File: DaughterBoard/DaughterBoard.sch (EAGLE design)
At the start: 6 parts

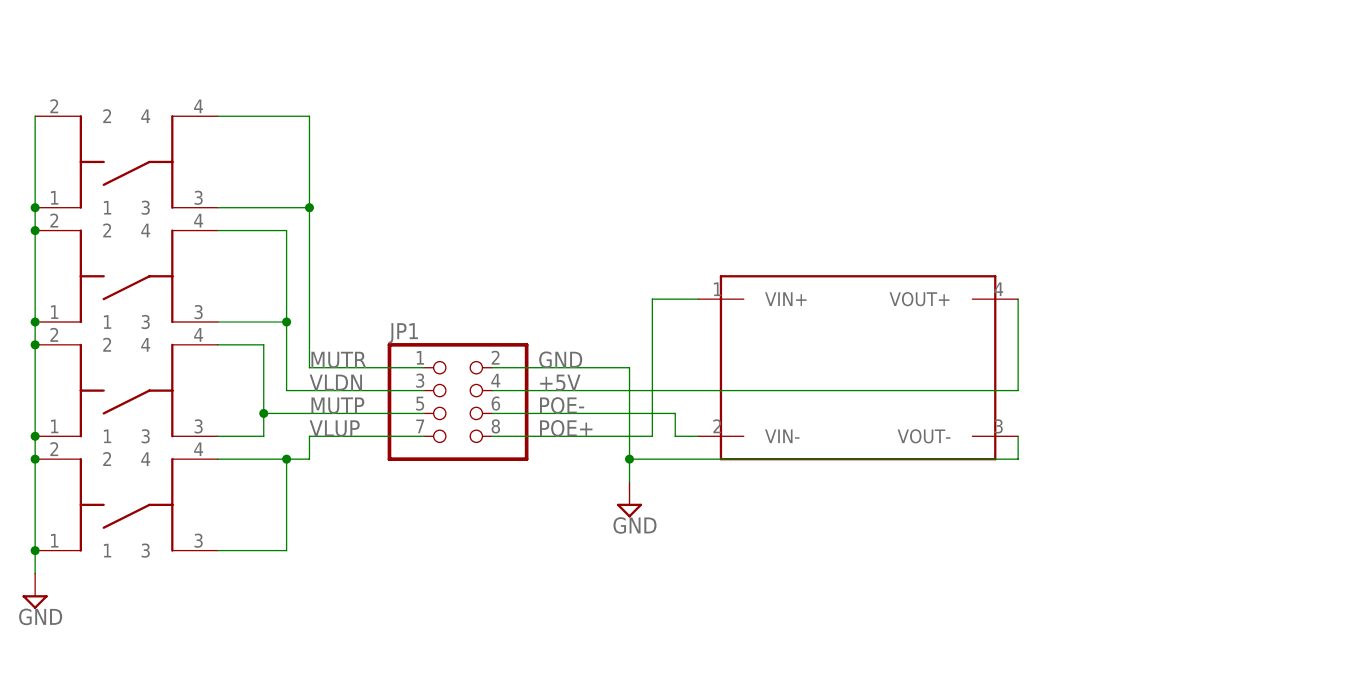
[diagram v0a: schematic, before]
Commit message: Finished modified daughterboard
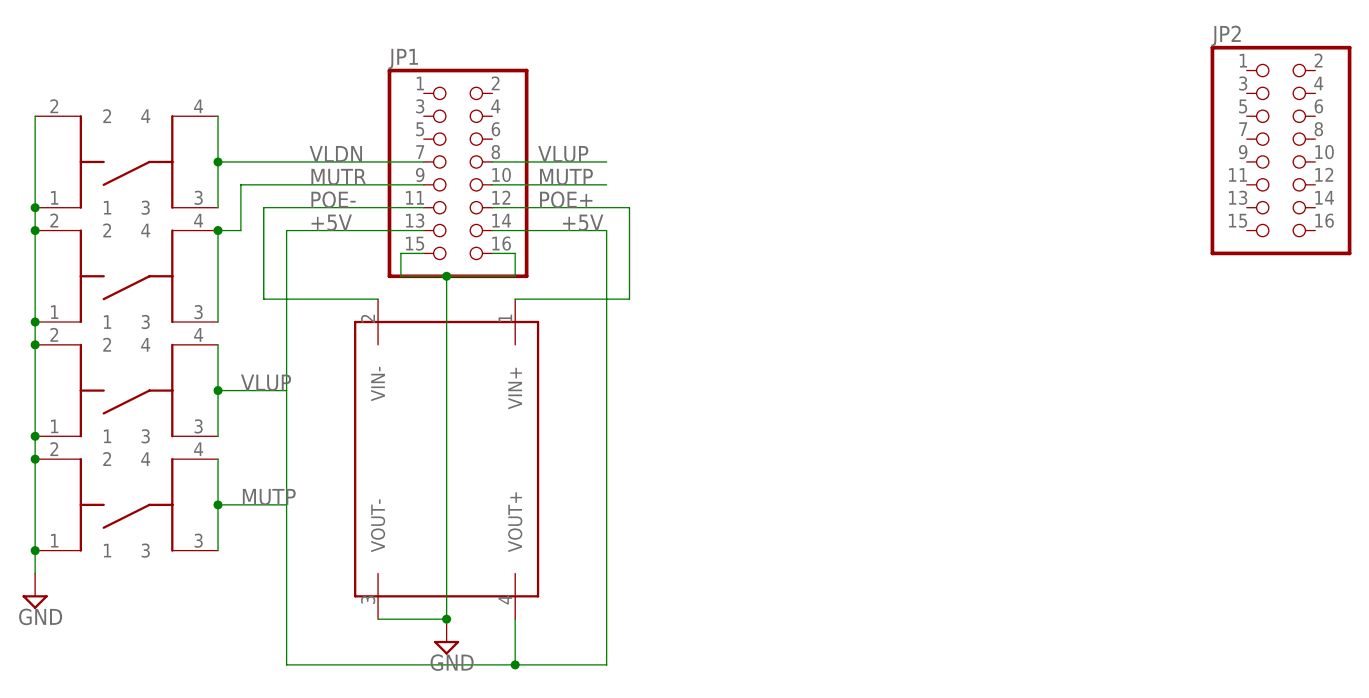
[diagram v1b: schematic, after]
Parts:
- added JP2: (no value), pinhead:PINHD-2X8
- JP1: device pinhead:PINHD-2X4 -> pinhead:PINHD-2X8
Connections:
- net +5V: now also JP1.13, JP1.14; no longer JP1.4
- net GND: now also JP1.15, JP1.16; no longer JP1.2
- net MUTP: now also JP1.10, U$5.3, U$5.4; no longer JP1.5, U$4.3, U$4.4
- net MUTR: now also JP1.9, U$3.3, U$3.4; no longer JP1.1, U$2.3, U$2.4
- net POE+: now also JP1.12; no longer JP1.8
- net POE-: now also JP1.11; no longer JP1.6
- net VLDN: now also JP1.7, U$2.3, U$2.4; no longer JP1.3, U$3.3, U$3.4
- net VLUP: now also JP1.8, U$4.3, U$4.4; no longer JP1.7, U$5.3, U$5.4
